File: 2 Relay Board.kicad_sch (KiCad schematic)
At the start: 42 parts, among them J1 Conn_01x02, J2 Conn_01x03, J3 Conn_01x05, K1 RAYEX-L90, K2 RAYEX-L90, Q1 BD139, Q2 BD139, U1 N76E003, U3 LM7809_TO220, U4 AMS1117-5.0, U5 CA56-12EWA, U6 CA56-12EWA

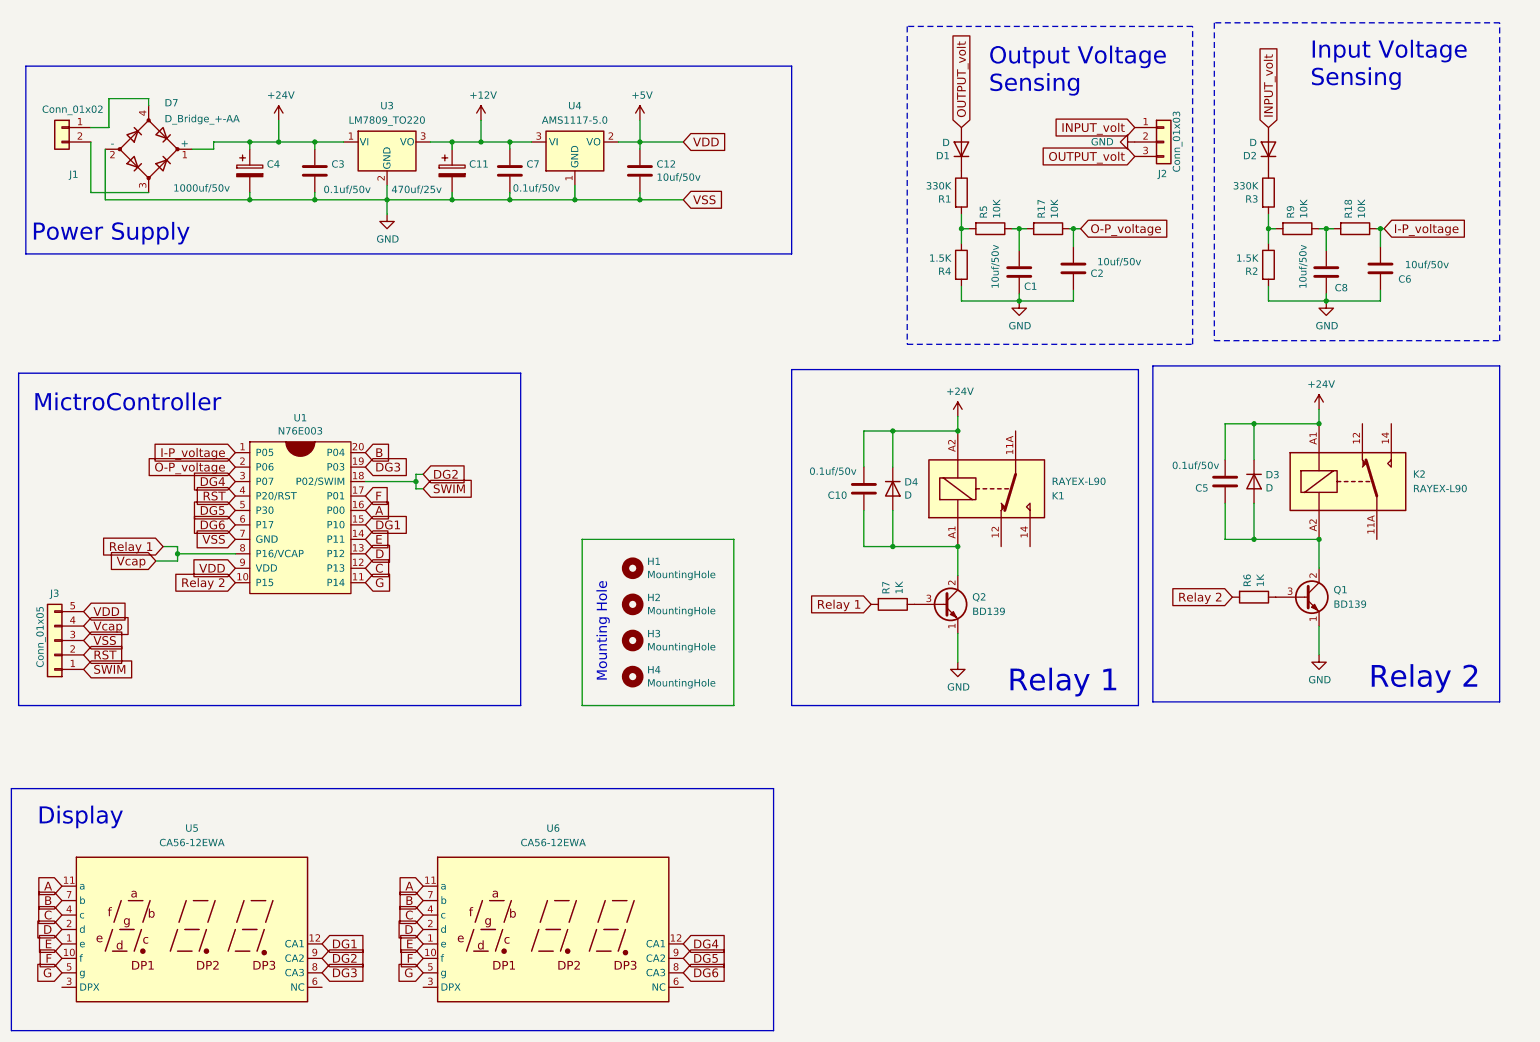
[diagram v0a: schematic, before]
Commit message: this version hase small 7805 v1.1
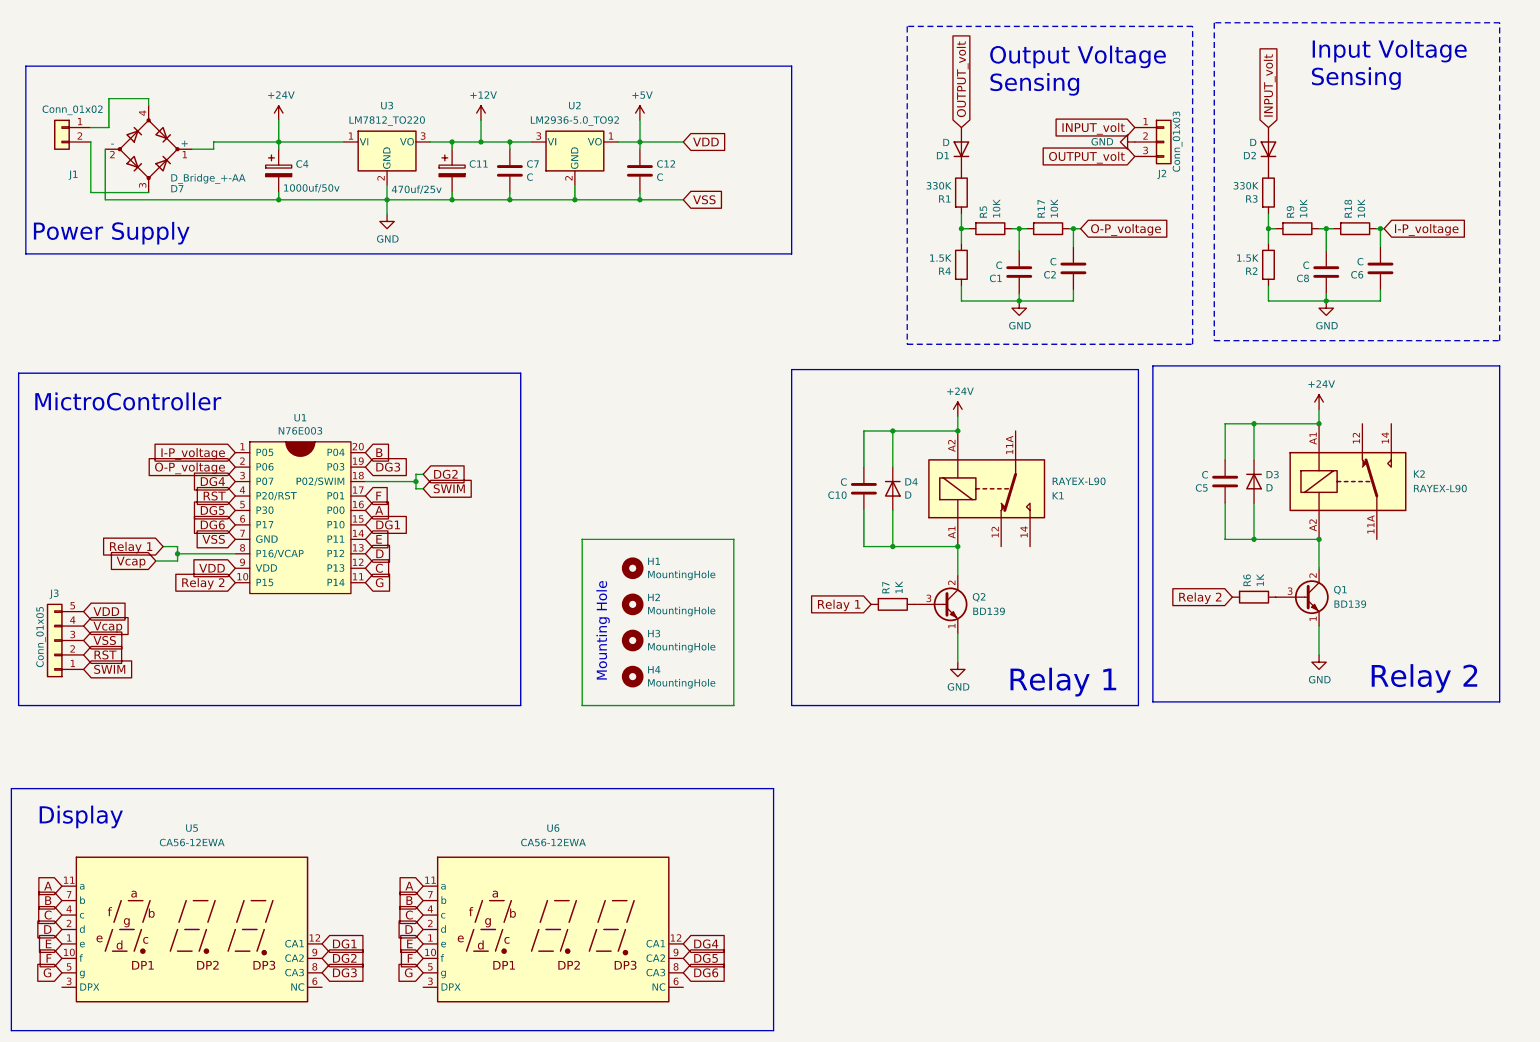
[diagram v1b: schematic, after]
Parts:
- removed C3: 0.1uf/50v, My Custom Footprint:C_1206_3216Metric, symbol Device:C
- removed U4: AMS1117-5.0, Package_TO_SOT_SMD:SOT-223-3_TabPin2, symbol Regulator_Linear:AMS1117-5.0
- added U2: LM2936-5.0_TO92, My Custom Footprint:TO-92_Inline_Wide_LM78L05, symbol Regulator_Linear:LM2936-5.0_TO92
- C1, C12, C2, C6, C8: value 10uf/50v -> C
- C10, C5, C7: value 0.1uf/50v -> C
- U3: value LM7809_TO220 -> LM7812_TO220
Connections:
- net +12V: now also U2.3 (VI)
- net +5V: now also U2.1 (VO)
- net GND: now also U2.2 (GND)
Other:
- moved on the sheet: C4

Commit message: this version hase smd LDO v1.2
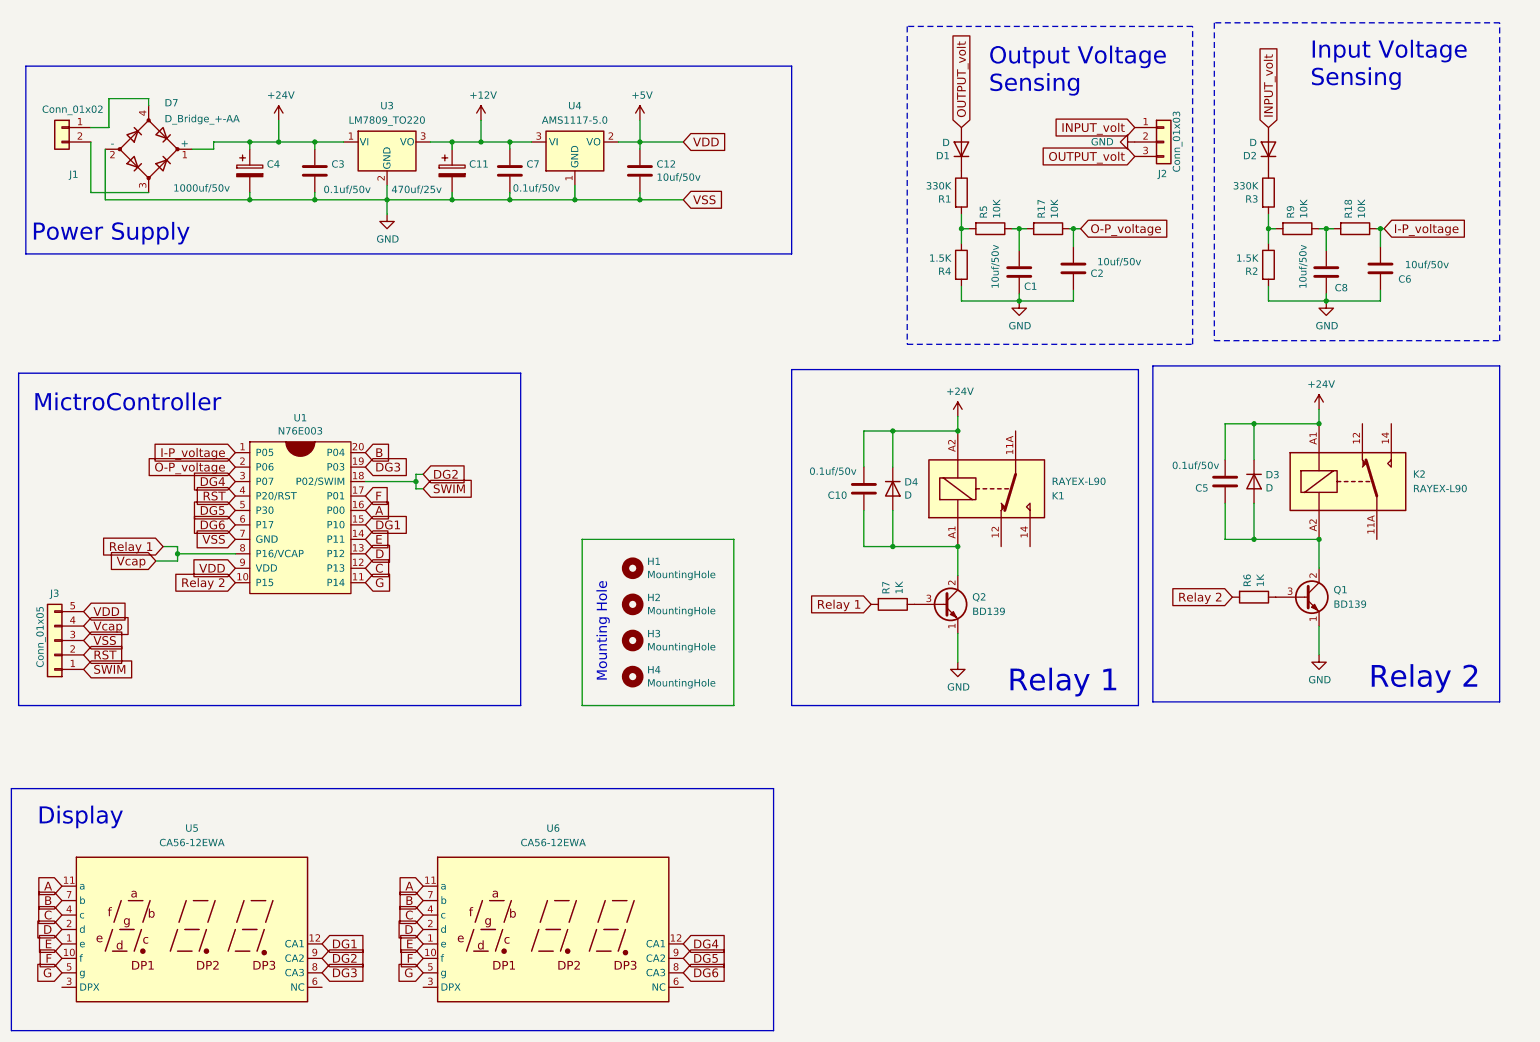
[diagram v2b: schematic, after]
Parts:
- removed U2: LM2936-5.0_TO92, My Custom Footprint:TO-92_Inline_Wide_LM78L05, symbol Regulator_Linear:LM2936-5.0_TO92
- added C3: 0.1uf/50v, My Custom Footprint:C_1206_3216Metric, symbol Device:C
- added U4: AMS1117-5.0, Package_TO_SOT_SMD:SOT-223-3_TabPin2, symbol Regulator_Linear:AMS1117-5.0
- C1, C12, C2, C6, C8: value C -> 10uf/50v
- C10, C5, C7: value C -> 0.1uf/50v
- U3: value LM7812_TO220 -> LM7809_TO220
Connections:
- net +12V: now also U4.3 (VI)
- net +24V: now also C3.2
- net +5V: now also U4.2 (VO)
- net GND: now also C3.1, U4.1 (GND)
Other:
- moved on the sheet: C4
